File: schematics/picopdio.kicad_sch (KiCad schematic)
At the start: 14 parts, among them J2 SWD+UART, J3 AudioJack3, SW1 Builtin Front Power Switch, SW2 Builtin Rear Power Switch, U1 MXA-10C_IR_Adapter_Main_Board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, U2 Pico, U3 Adafruit_VS1053B_Breakout, U4 W5500_Lite USR-ES1, U5 MCP23017_SP, U6 SparkFun_SX1509_Expander, U7 Pololu_2808

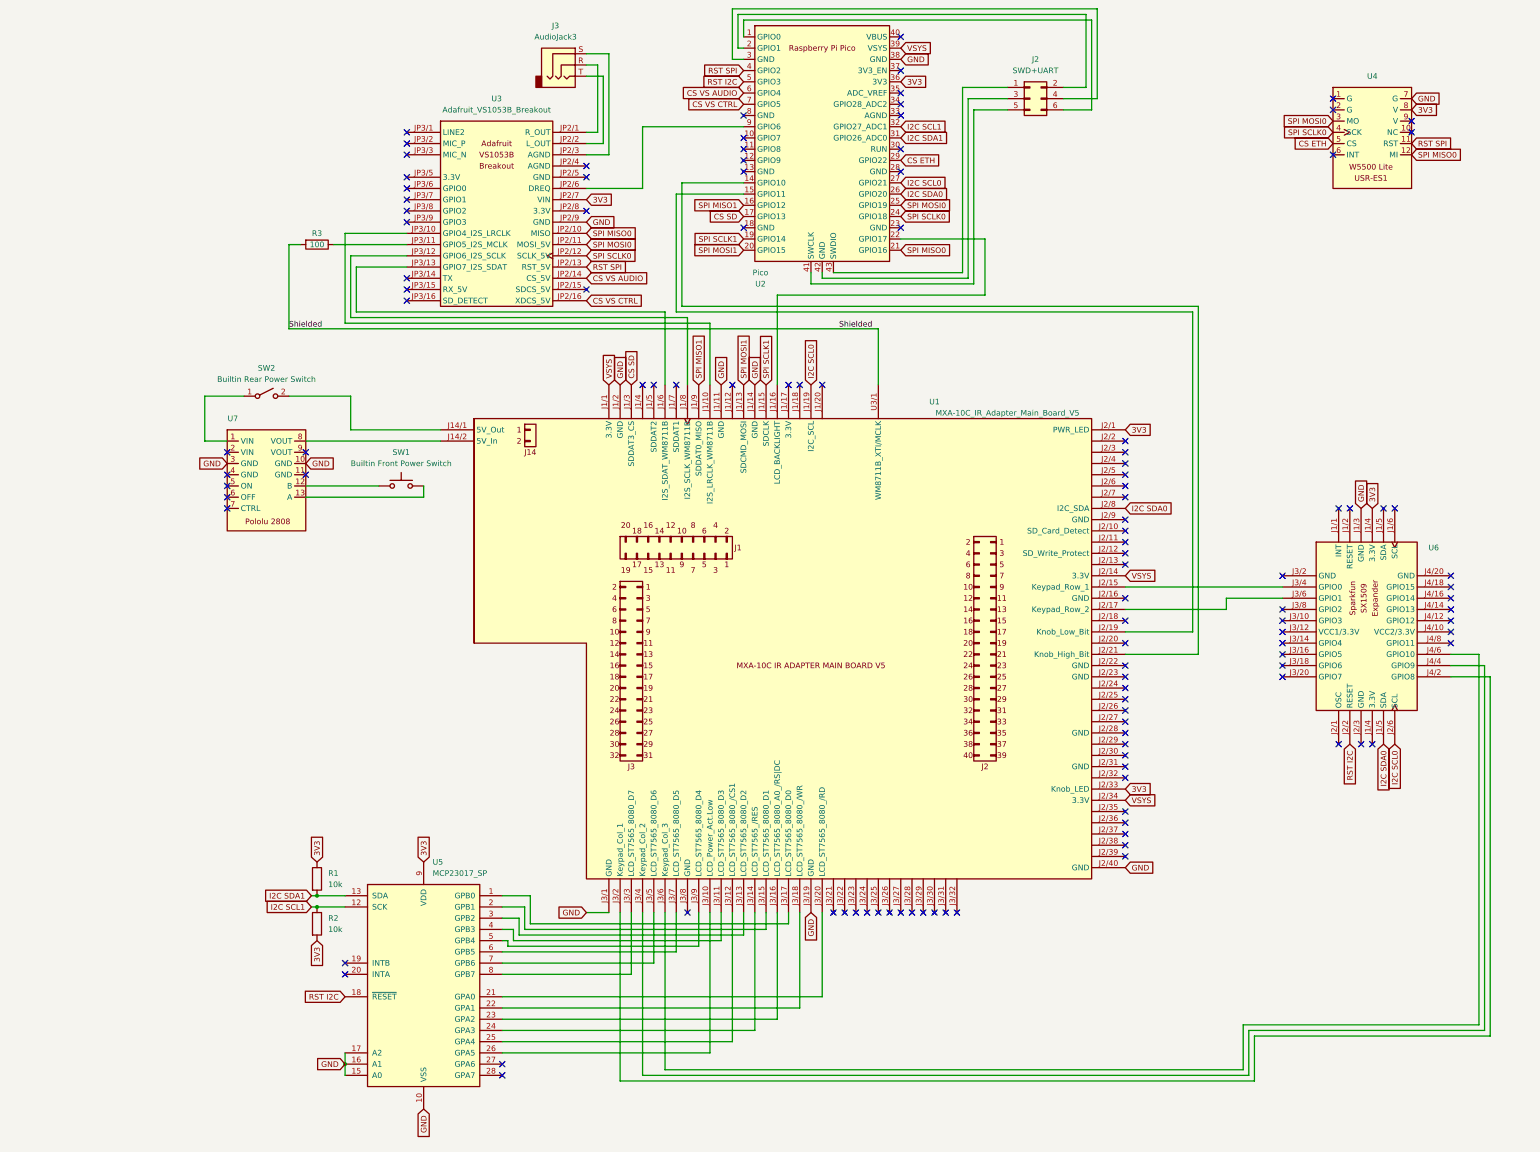
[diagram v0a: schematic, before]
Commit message: wip
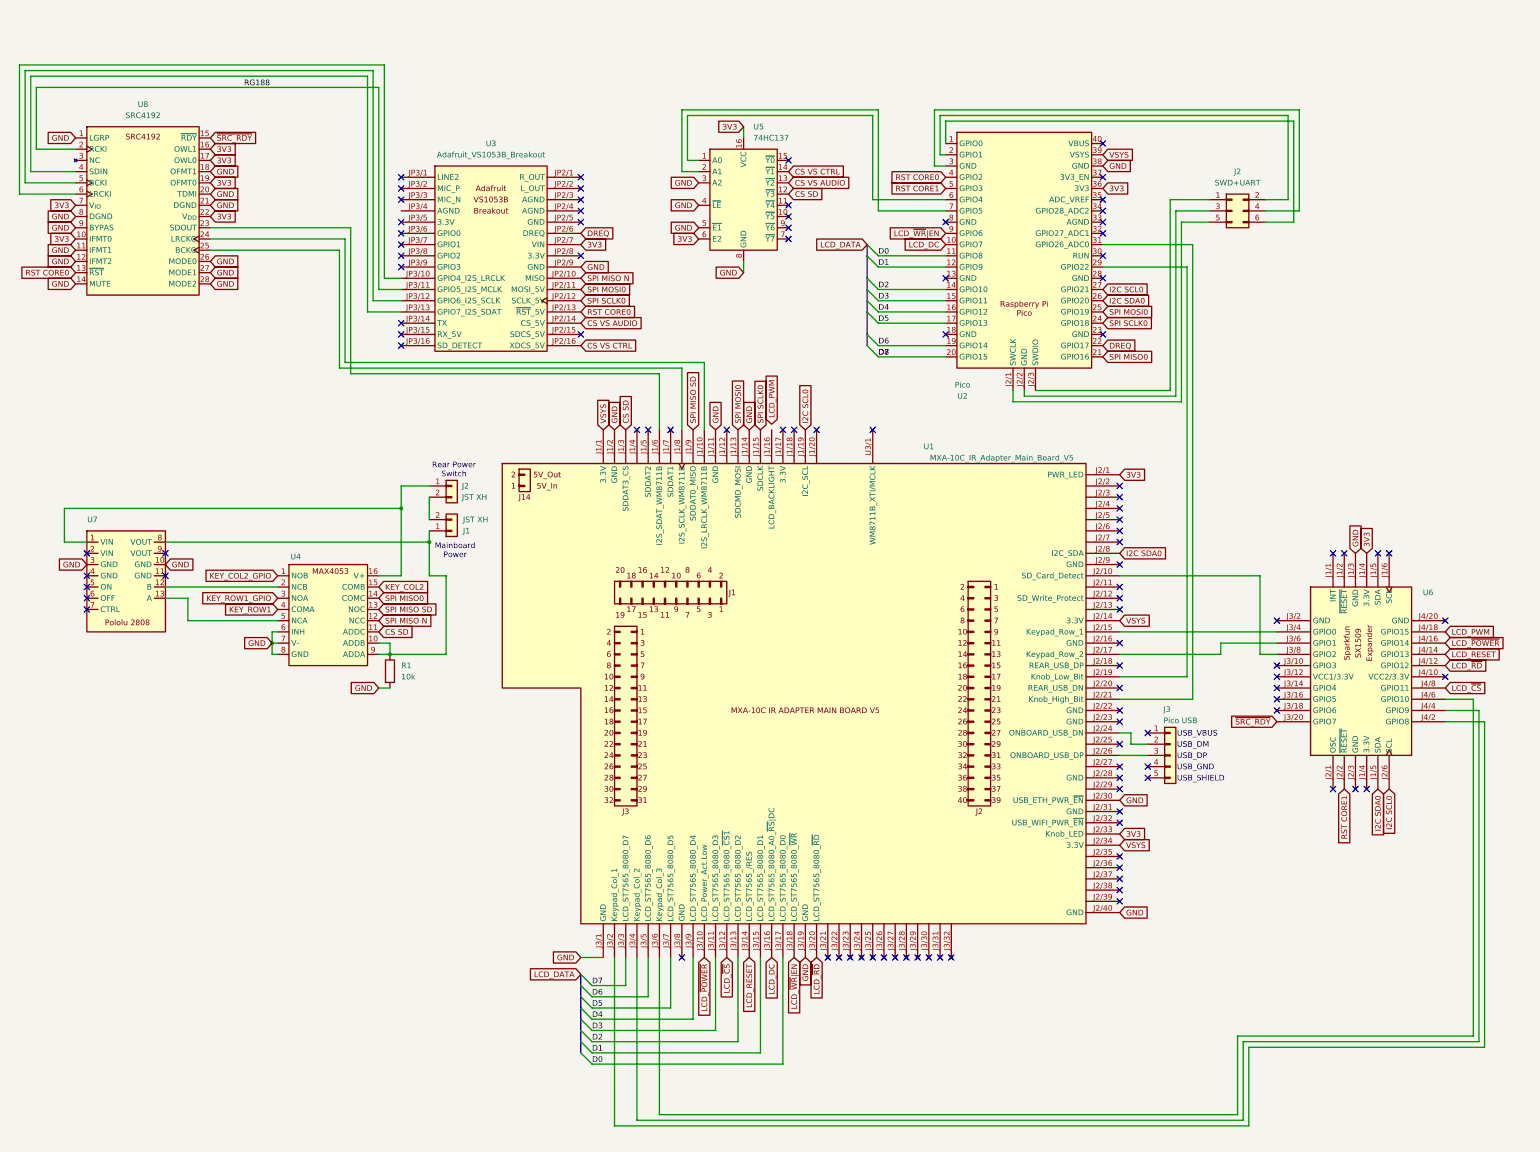
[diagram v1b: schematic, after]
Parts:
- removed J3: AudioJack3, symbol Connector:AudioJack3
- removed R2: 10k, symbol Device:R
- removed R3: 100, symbol Device:R
- removed SW1: Builtin Front Power Switch, symbol Switch:SW_Push
- removed SW2: Builtin Rear Power Switch, symbol Switch:SW_SPST
- removed U4: W5500_Lite USR-ES1, symbol picopdio:W5500_Lite USR-ES1
- removed U5: MCP23017_SP, Package_DIP:DIP-28_W7.62mm, symbol Interface_Expansion:MCP23017_SP
- added J1, J2: JST XH, symbol Connector_Generic:Conn_01x02
- added J3: Pico USB, symbol Connector_Generic:Conn_01x05
- added U4: ~, symbol picopdio:MAX4053
- added U5: 74HC137, symbol 74xx:74HC137
- added U8: SRC4192, Package_SO:SSOP-28_5.3x10.2mm_P0.65mm, symbol picopdio:SRC4192
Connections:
- net CS ETH is gone; now on an unnamed net: U2.29 (GPIO22)
- net 3V3: now also U5.16 (VCC), U5.6 (E2), U8.10 (IFMT0), U8.16 (OWL1), U8.17 (OWL0), U8.19 (OFMT0), U8.22 (V_{DD}), U8.7 (V_{IO}); no longer R1.1
- net CS SD: now also U4.11 (ADDC), U5.12 (~{Y3}); no longer U2.17 (GPIO13)
- net CS VS AUDIO: now also U5.13 (~{Y2}); no longer U2.6 (GPIO4)
- net CS VS CTRL: now also U5.14 (~{Y1}); no longer U2.7 (GPIO5)
- net GND: now also R1.2, U1.J2/30 (USB_ETH_PWR_~{EN}), U4.6 (INH), U4.7 (V-), U4.8 (GND), U5.3 (A2), U5.4 (~{LE}), U5.5 (~{E1}), U5.8 (GND), U8.1 (LGRP), U8.11 (IFMT1), U8.12 (IFMT2), U8.14 (MUTE), U8.18 (OFMT1), U8.20 (TDMI), U8.21 (DGND), U8.26 (MODE0), U8.27 (MODE1), U8.28 (MODE2), U8.8 (DGND), U8.9 (BYPAS)
- net SPI MISO0: now also U4.14 (COMC); no longer U3.JP2/10 (MISO)
- net SPI MOSI0: now also U1.J1/13 (SDCMD_MOSI)
- net SPI SCLK0: now also U1.J1/15 (SDCLK)
- net RG188: now reaches U3.JP3/11 (GPIO5_I2S_MCLK)
- net RG188: now also U8.2 (RCKI)
- net at J2.1 (Pin_1): now also U2.J2/3 (SWDIO); no longer U2.43 (SWDIO)
- net at J2.3 (Pin_3): now also U2.J2/2 (GND); no longer U2.42 (GND)
- net at J2.5 (Pin_5): now also U2.J2/1 (SWCLK); no longer U2.41 (SWCLK)
- net at U1.J1/10 (I2S_LRCLK_WM8711B): now also U8.24 (LRCKO); no longer U3.JP3/10 (GPIO4_I2S_LRCLK)
- net at U1.J1/16 (LCD_BACKLIGHT): no longer U2.22 (GPIO17)
- net at U1.J1/6 (I2S_SDAT_WM8711B): now also U8.23 (SDOUT); no longer U3.JP3/13 (GPIO7_I2S_SDAT)
- net at U1.J1/8 (I2S_SCLK_WM8711B): now also U8.25 (BCKO); no longer U3.JP3/12 (GPIO6_I2S_SCLK)
- net at U7.8 (VOUT): now also R1.1, J1.1 (Pin_1), U4.10 (ADDB), U4.9 (ADDA); no longer U1.J14/2 (5V_In)
- net at U1.J2/10 (SD_Card_Detect): now also U6.J3/8 (GPIO2)
- net at U1.J2/19 (Knob_Low_Bit): no longer U2.15 (GPIO11)
- net at U1.J2/21 (Knob_High_Bit): now also U2.31 (GPIO26_ADC0); no longer U2.14 (GPIO10)
- net at U1.J2/24 (ONBOARD_USB_DN): now also J3.2 (Pin_2)
- net at U1.J2/26 (ONBOARD_USB_DP): now also J3.3 (Pin_3)
- net LCD_~{POWER}: now reaches U1.J3/10 (LCD_Power_Act.Low)
- net LCD_~{POWER}: now also U6.J4/16 (GPIO14)
- net D3: now reaches U1.J3/11 (LCD_ST7565_8080_D3)
- net D3: now also U2.15 (GPIO11)
- net LCD_~{CS}: now reaches U1.J3/12 (LCD_ST7565_8080_~{CS1})
- net LCD_~{CS}: now also U6.J4/8 (GPIO11)
- net D2: now reaches U1.J3/13 (LCD_ST7565_8080_D2)
- net D2: now also U2.14 (GPIO10)
- net LCD_RESET: now reaches U1.J3/14 (LCD_ST7565_/RES)
- net LCD_RESET: now also U6.J4/14 (GPIO13)
- net D1: now reaches U1.J3/15 (LCD_ST7565_8080_D1)
- net D1: now also U2.12 (GPIO9)
- net LCD_DC: now reaches U1.J3/16 (LCD_ST7565_8080_A0_~{RS}|DC)
- net LCD_DC: now also U2.10 (GPIO7)
- net D0: now reaches U1.J3/17 (LCD_ST7565_8080_D0)
- net D0: now also U2.11 (GPIO8)
- net LCD_~{WR}|EN: now reaches U1.J3/18 (LCD_ST7565_8080_~{WR})
- net LCD_~{WR}|EN: now also U2.9 (GPIO6)
- net LCD_~{RD}: now reaches U1.J3/20 (LCD_ST7565_8080_~{RD})
- net LCD_~{RD}: now also U6.J4/12 (GPIO12)
- net D7: now reaches U1.J3/3 (LCD_ST7565_8080_D7)
- net D7: now also U2.20 (GPIO15)
- net D6: now reaches U1.J3/5 (LCD_ST7565_8080_D6)
- net D6: now also U2.19 (GPIO14)
- net D5: now reaches U1.J3/7 (LCD_ST7565_8080_D5)
- net D5: now also U2.17 (GPIO13)
- net D4: now reaches U1.J3/9 (LCD_ST7565_8080_D4)
- net D4: now also U2.16 (GPIO12)
- net DREQ: now reaches U3.JP2/6 (DREQ)
- net DREQ: now also U2.22 (GPIO17); no longer U2.9 (GPIO6)
- net at U7.12 (B): now also U4.2 (NCB)
- net at U7.13 (A): now also U4.5 (NCA)
- net ~{SRC_RDY}: now reaches U6.J3/20 (GPIO7)
- net ~{SRC_RDY}: now also U8.15 (~{RDY})
- net LCD_PWM: now reaches U6.J4/18 (GPIO15)
- net at U7.1 (VIN): now also J2.1 (Pin_1), U4.16 (V+)
- net I2C SCL1: no longer names the net of U2.32 (GPIO27_ADC1)
- removed net I2C SDA1: R1.2, U2.31 (GPIO26_ADC0)
- net RST I2C renamed RST CORE1
- net RST SPI renamed RST CORE0
- net RST CORE0: now also U8.13 (~{RST})
- net SPI MISO1 renamed SPI MISO SD
- net SPI MISO SD: now also U4.13 (NOC); no longer U2.16 (GPIO12)
- removed net SPI MOSI1: U1.J1/13 (SDCMD_MOSI), U2.20 (GPIO15)
- removed net SPI SCLK1: U1.J1/15 (SDCLK), U2.19 (GPIO14)
- net Shielded: no longer names the net of U1.U3/1 (WM8711B_XTI/MCLK)
- new net: U2.6 (GPIO4), U5.1 (A0)
- new net: U2.7 (GPIO5), U5.2 (A1)
- new net: U3.JP3/10 (GPIO4_I2S_LRCLK), U8.6 (LRCKI)
- new net: U3.JP3/12 (GPIO6_I2S_SCLK), U8.5 (BCKI)
- new net: U3.JP3/13 (GPIO7_I2S_SDAT), U8.4 (SDIN)
- new net: J1.2 (Pin_2), J2.2 (Pin_2)
- new net KEY_COL2: U4.15 (COMB)
- new net KEY_COL2_GPIO: U4.1 (NOB)
- new net KEY_ROW1: U4.4 (COMA)
- new net KEY_ROW1_GPIO: U4.3 (NOA)
- new net SPI MISO N: U3.JP2/10 (MISO), U4.12 (NCC)
- no-connect marks 117 -> 107
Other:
- note added: "Mainboard Power"
- note added: "Rear Power Switch"
- note added: "USB_DM"
- note added: "USB_DP"
- note added: "USB_GND"
- note added: "USB_SHIELD"
- note added: "USB_VBUS"
- moved on the sheet: J2, U6, U7
